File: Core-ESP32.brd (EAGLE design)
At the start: 149.8 x 80.5 mm, 63 parts, among them J3 CONNECTOR-GROVE-4P-2.0-347013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, Q1 BSS138, Q10 BSS138, Q11 BSS138, Q12 BSS138, Q13 BSS138, Q2 BSS138, Q3 BSS138, Q4 BSS138, Q5 BSS138, Q6 BSS138, Q7 BSS138, Q8 BSS138, Q9 BSS138

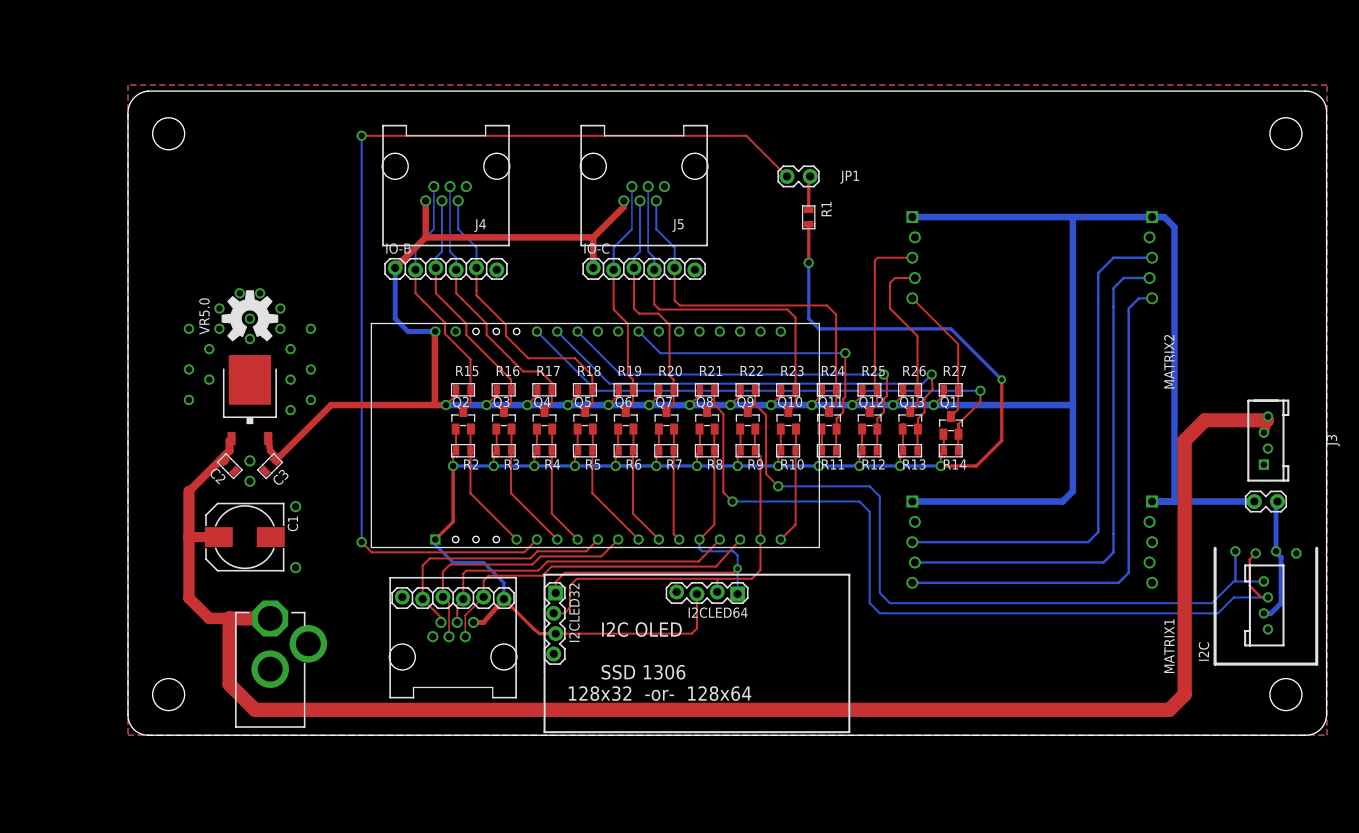
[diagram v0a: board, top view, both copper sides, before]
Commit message: 2.1
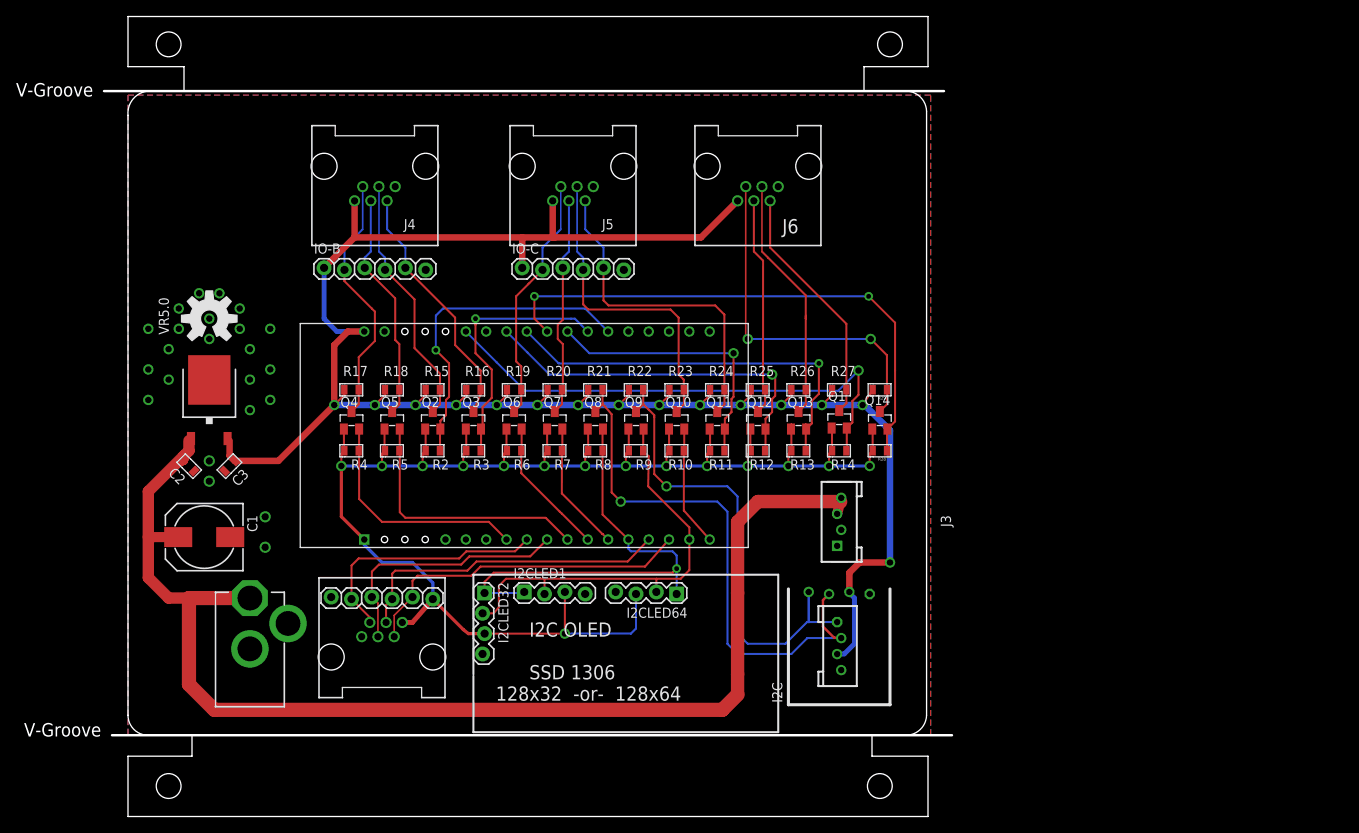
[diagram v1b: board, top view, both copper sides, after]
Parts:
- removed JP1: LED, SparkFun-Connectors:1X02_LOCK
- removed JP2: 5v I2C Power, SparkFun-Connectors:1X02_LOCK
- removed MATRIX1, MATRIX2: LEDMATRIX, SPCoast:LEDMATRIX
- removed R1: 220R, SPCoast:0805-RES
- added I2CLED1: (no value), SPCoast:1X04_LOCK
- added J6: (no value), SPCoast:RJ25-INVERTED
- added Q14: BSS138, SPCoast:SOT23
- added R28, R29: 10k, SPCoast:0805-RES
- BOARD: device SPCoast:BOARD-DINRAIL-3.17INX15CM -> SPCoast:BOARD-DINRAIL-3.17IN-NOHOLES
- moved J3 54.3 mm to (88.9, 26.7)
- moved I2C 53.6 mm to (88.9, 17.8)
- moved Q4 24.1 mm to (27.9, 39.4)
- moved R17 24.1 mm to (27.9, 43.2)
- moved R4 24.1 mm to (27.9, 35.6)
- moved Q5 24.1 mm to (33.0, 39.4)
- moved R18 24.1 mm to (33.0, 43.2)
- moved R5 24.1 mm to (33.0, 35.6)
- moved Q1 14.0 mm to (88.9, 39.5)
- moved Q13 14.0 mm to (83.8, 39.4)
- moved R13 14.0 mm to (83.8, 35.6)
- moved R26 14.0 mm to (83.8, 43.2)
- moved Q10 14.0 mm to (68.6, 39.4)
- moved Q11 14.0 mm to (73.7, 39.4)
- moved Q12 14.0 mm to (78.7, 39.4)
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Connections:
- removed net D0H: IO-B.2, J4.2, Q2.3, R15.1
- removed net D12H: MATRIX2.CS@1, Q13.3, R26.1
- removed net D2H: IO-B.3, J4.3, Q3.3, R16.1
- removed net N$1: JP1.1, R1.1
- removed net N$10: MATRIX1.CLK@1, MATRIX2.CLK@2
- removed net N$3: MATRIX1.DI, MATRIX2.DO
- removed net N$44: I2C.V+, I2C.V+@1, JP2.1
- removed net N$9: MATRIX1.CS@1, MATRIX2.CS@2
- new net D26H: J6.2, Q14.3, R29.1
- new net D27H: J6.4, Q13.3, R26.1
- new net D32H: IO-B.4, J4.4, Q2.3, R15.1
- new net D33H: IO-B.5, J4.5, Q3.3, R16.1
- net +3V3: now also I2CLED1.3, Q14.1, R28.2; no longer R1.2
- net D0: no longer Q2.2, R2.1
- net D12: no longer Q13.2, R13.1
- net D13H: now also J6.5; no longer MATRIX2.CLK@1
- net D14H: now also J6.3; no longer MATRIX2.DI
- net D15: no longer JP1.2
- net D2: no longer Q3.2, R3.1
- net D26: now also Q14.2, R28.1
- net D27: now also Q13.2, R13.1
- net D32: now also Q2.2, R2.1
- net D33: now also Q3.2, R3.1
- net D4H: now also IO-B.2, J4.2; no longer IO-B.4, J4.4
- net D5H: now also IO-B.3, J4.3; no longer IO-B.5, J4.5
- net GND: now also I2CLED1.4, J6.6; no longer MATRIX1.G@1, MATRIX1.G@2, MATRIX2.G@1, MATRIX2.G@2
- net SCL: now also I2CLED1.2
- net SDA: now also I2CLED1.1
- net VCCIO: now also I2C.V+, I2C.V+@1, J6.1, R29.2; no longer JP2.2, MATRIX1.V+@1, MATRIX1.V+@2, MATRIX2.V+@1, MATRIX2.V+@2
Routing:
- net D15: track 129.2 -> 0.00 mm, vias 2 -> 0
- net VCCIO: track 338.4 -> 249.5 mm, vias 13 -> 15
- net D26: track 0.00 -> 67.9 mm, vias 0 -> 2
- net N$10: track 64.0 -> 0.00 mm
- net N$3: track 63.7 -> 0.00 mm
- net N$9: track 63.4 -> 0.00 mm
- net D12: track 61.4 -> 0.00 mm, vias 1 -> 0
- net +9V: track 212.8 -> 156.9 mm
- net D27: track 0.00 -> 50.9 mm, vias 0 -> 1
- net D26H: track 0.00 -> 45.0 mm, vias 0 -> 2
- net D32: track 0.00 -> 41.1 mm, vias 0 -> 1
- net +3V3: track 238.3 -> 200.1 mm
- net SDAH: track 103.8 -> 69.5 mm
- net SCLH: track 93.3 -> 59.0 mm
- net D33: track 0.00 -> 32.6 mm, vias 0 -> 1
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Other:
- board size 149.8 x 80.5 mm -> 106 x 100 mm
- board text added: "2018.07"
- board text added: "CS"
- board text added: "Clk"
- board text added: "D13"
- board text added: "D14"
- board text added: "D26"
- board text added: "D27"
- board text added: "D32"
- board text added: "D33"
- board text added: "Data"
- board text added: "Geekcreit ESP32 WROOM"
- board text added: "IO1"
- board text added: "v2.1"
- board text removed: "+"
- board text removed: "-"
- board text removed: "2018.05"
- board text removed: "CS D12"
- board text removed: "Clock D13"
- board text removed: "D0"
- board text removed: "D15 LED"
- board text removed: "D2"
- board text removed: "Data D14"
- board text removed: "Geekcreit ESP32"
- board text removed: "v2.0"
